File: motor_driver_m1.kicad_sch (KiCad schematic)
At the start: 32 parts, among them J4 Conn_01x01_Pin, J5 Conn_01x01_Pin, J6 Conn_01x01_Pin, M1 DRV8320SRTVR, Q1 NP80N06D6, Q2 NP80N06D6, Q3 NP80N06D6, Q4 NP80N06D6, Q5 NP80N06D6, Q6 NP80N06D6

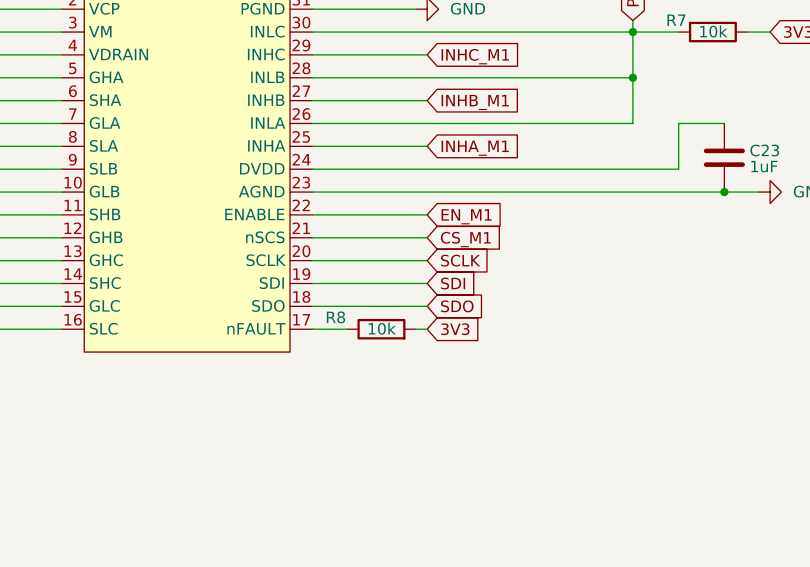
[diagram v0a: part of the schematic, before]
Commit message: ...
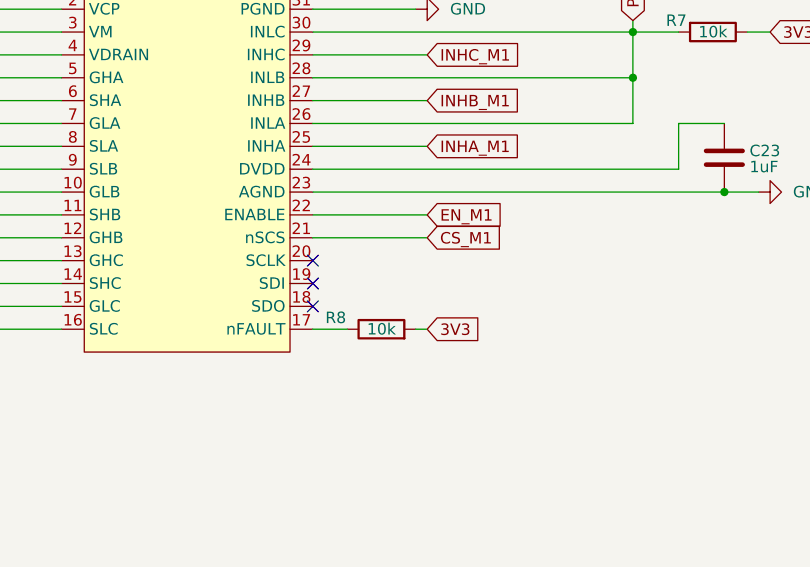
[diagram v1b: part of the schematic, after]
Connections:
- net SCLK: no longer names the net of M1.20 (SCLK)
- net SDI: no longer names the net of M1.19 (SDI)
- net SDO: no longer names the net of M1.18 (SDO)
- no-connect marks 0 -> 3
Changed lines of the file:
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@@
 		(color 0 0 0 0)
 	)
+	(no_connect
+		(at 96.52 76.2)
+	)
+	(no_connect
+		(at 96.52 71.12)
+	)
+	(no_connect
+		(at 96.52 73.66)
+	)
 	(wire
 		(pts
@@
 	(wire
 		(pts
-			(xy 96.52 76.2) (xy 109.22 76.2)
-		)
-		(stroke
-			(width 0)
-			(type default)
-		)
-	)
-	(wire
-		(pts
 			(xy 85.09 182.88) (xy 85.09 184.15)
 		)
@@
 	(wire
 		(pts
-			(xy 109.22 71.12) (xy 96.52 71.12)
-		)
-		(stroke
-			(width 0)
-			(type default)
-		)
-	)
-	(wire
-		(pts
 			(xy 40.64 182.88) (xy 40.64 184.15)
 		)
@@
 	(wire
 		(pts
-			(xy 109.22 73.66) (xy 96.52 73.66)
-		)
-		(stroke
-			(width 0)
-			(type default)
-		)
-	)
-	(wire
-		(pts
 			(xy 214.63 73.66) (xy 223.52 73.66)
 		)
@@
 		)
 	)
-	(global_label "SDI"
-		(shape input)
-		(at 109.22 73.66 0)
-		(fields_autoplaced yes)
-		(effects
-			(font
-				(size 1.27 1.27)
-			)
-			(justify left)
-		)
-		(property "Intersheetrefs" "${INTERSHEET_REFS}"
-			(at 115.2895 73.66 0)
-			(effects
-				(font
-					(size 1.27 1.27)
-				)
-				(justify left)
-				(hide yes)
-			)
-		)
-	)
 	(global_label "GLC1"
 		(shape input)
@@
 		)
 	)
-	(global_label "SDO"
-		(shape input)
-		(at 109.22 76.2 0)
-		(fields_autoplaced yes)
-		(effects
-			(font
-				(size 1.27 1.27)
-			)
-			(justify left)
-		)
-		(property "Intersheetrefs" "${INTERSHEET_REFS}"
-			(at 116.0152 76.2 0)
-			(effects
-				(font
-					(size 1.27 1.27)
-				)
-				(justify left)
-				(hide yes)
-			)
-		)
-	)
 	(global_label "SHC1"
 		(shape input)
@@
 			(effects
 				(font
-					(size 1.27 1.27)
-				)
-				(justify left)
-				(hide yes)
-			)
-		)
-	)
-	(global_label "SCLK"
-		(shape input)
-		(at 109.22 71.12 0)
-		(fields_autoplaced yes)
-		(effects
-			(font
-				(size 1.27 1.27)
-			)
-			(justify left)
-		)
-		(property "Intersheetrefs" "${INTERSHEET_REFS}"
-			(at 116.9828 71.12 0)
-			(effects
-				(font
